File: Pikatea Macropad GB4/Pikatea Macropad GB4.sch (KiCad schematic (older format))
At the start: 30 parts, among them J1 AVR-ISP-6, J2 USB_B_Mini, J3 Conn_01x03_Male, J4 Conn_01x03_Male, J5 Conn_01x03_Male, J6 Conn_01x06_Male, J7 Conn_01x03_Male, SW1 SW_DPST, SW2 Rotary_Encoder_Switch, U1 ATMEGA32U4-EP, X1 16MHz

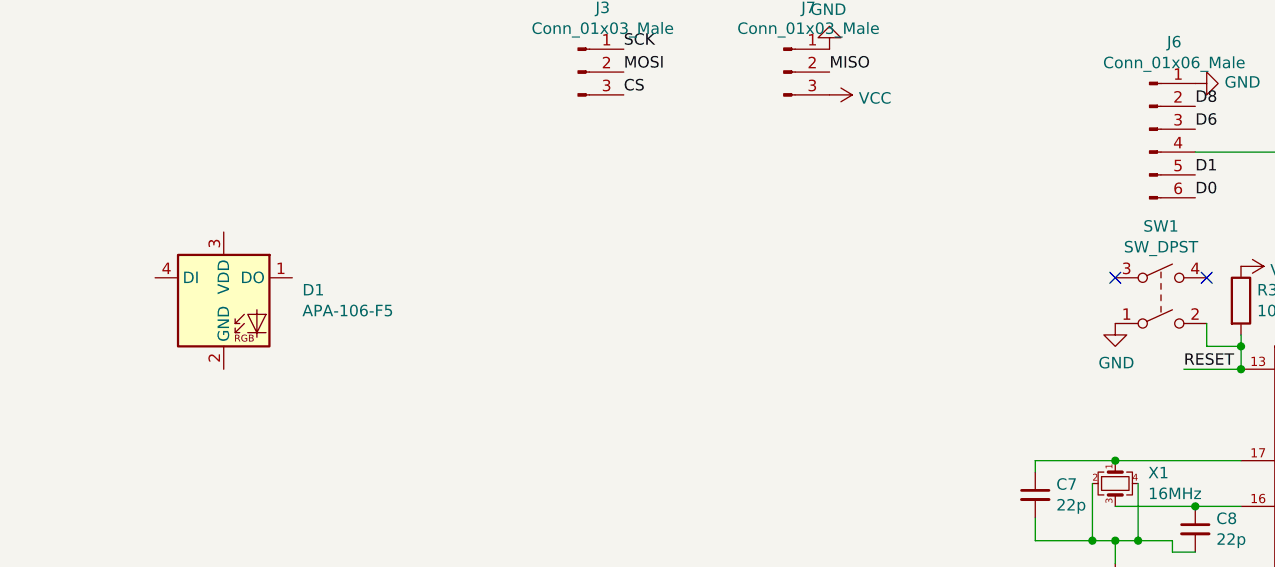
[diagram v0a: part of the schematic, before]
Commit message: update GB4
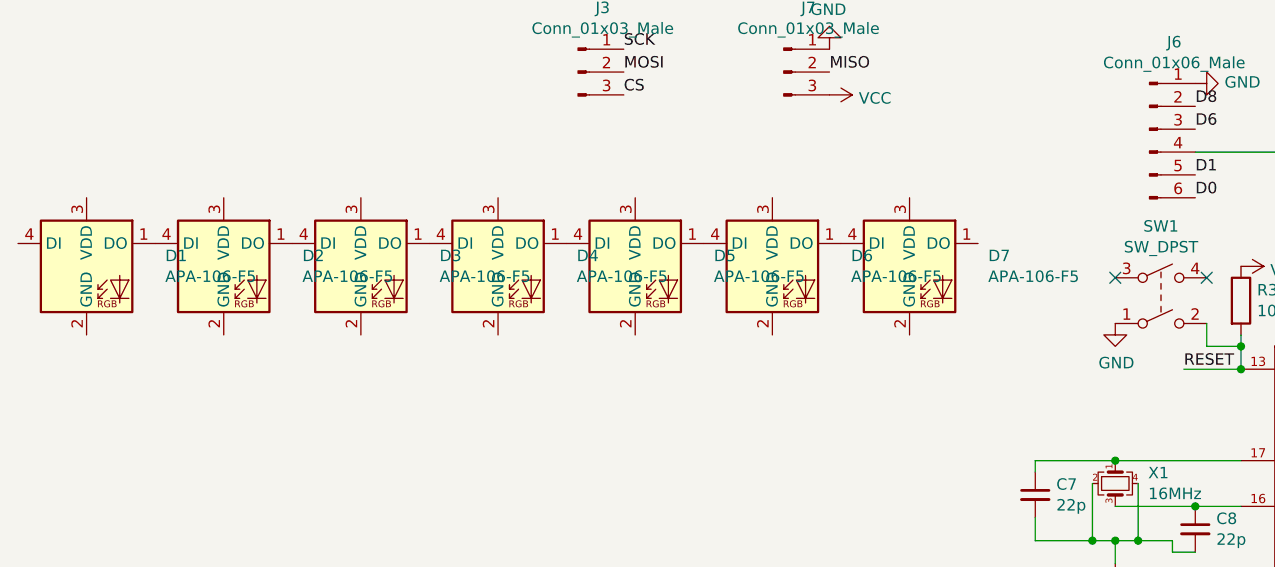
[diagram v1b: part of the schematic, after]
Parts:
- added D2, D3, D4, D5, D6, D7: APA-106-F5, Pikatea:TONYU-DY-S352818-RGBC, symbol LED:APA-106-F5
- D1: footprint LED_THT:LED_D5.0mm-4_RGB -> Pikatea:TONYU-DY-S352818-RGBC
- MX1, MX2, MX3, MX4, MX5: footprint MX_Only:MXOnly-1U -> MX_Only:MXOnly-1U-NoLED
- U1: footprint Package_QFP:LQFP-44_10x10mm_P0.8mm -> Package_DFN_QFN:QFN-44-1EP_7x7mm_P0.5mm_EP5.15x5.15mm_ThermalVias
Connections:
- net at D1.1 (DO): now also D2.4 (DI)
- new net: D2.1 (DO), D3.4 (DI)
- new net: D3.1 (DO), D4.4 (DI)
- new net: D4.1 (DO), D5.4 (DI)
- new net: D5.1 (DO), D6.4 (DI)
- new net: D6.1 (DO), D7.4 (DI)
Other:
- moved on the sheet: D1
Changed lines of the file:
@@
 F 0 "U1" H 7075 6581 50  0000 C CNN
 F 1 "ATMEGA32U4-EP" H 7075 6490 50  0000 C CNN
-F 2 "Package_QFP:LQFP-44_10x10mm_P0.8mm" H 7100 4600 50  0001 C CIN
+F 2 "Package_DFN_QFN:QFN-44-1EP_7x7mm_P0.5mm_EP5.15x5.15mm_ThermalVias" H 7100 4600 50  0001 C CIN
 F 3 "" H 8200 5700 50  0001 C CNN
 	1    7100 4600
@@
 F 0 "MX1" H 7382 2074 60  0000 C CNN
 F 1 "MX-LED" H 7382 2000 20  0000 C CNN
-F 2 "MX_Only:MXOnly-1U" H 6675 1825 60  0001 C CNN
+F 2 "MX_Only:MXOnly-1U-NoLED" H 6675 1825 60  0001 C CNN
 F 3 "" H 6675 1825 60  0001 C CNN
 	1    7300 1850
@@
 F 0 "MX2" H 7832 2074 60  0000 C CNN
 F 1 "MX-LED" H 7832 2000 20  0000 C CNN
-F 2 "MX_Only:MXOnly-1U" H 7125 1825 60  0001 C CNN
+F 2 "MX_Only:MXOnly-1U-NoLED" H 7125 1825 60  0001 C CNN
 F 3 "" H 7125 1825 60  0001 C CNN
 	1    7750 1850
@@
 F 0 "MX3" H 8282 2074 60  0000 C CNN
 F 1 "MX-LED" H 8282 2000 20  0000 C CNN
-F 2 "MX_Only:MXOnly-1U" H 7575 1825 60  0001 C CNN
+F 2 "MX_Only:MXOnly-1U-NoLED" H 7575 1825 60  0001 C CNN
 F 3 "" H 7575 1825 60  0001 C CNN
 	1    8200 1850
@@
 F 0 "MX4" H 8732 2074 60  0000 C CNN
 F 1 "MX-LED" H 8732 2000 20  0000 C CNN
-F 2 "MX_Only:MXOnly-1U" H 8025 1825 60  0001 C CNN
+F 2 "MX_Only:MXOnly-1U-NoLED" H 8025 1825 60  0001 C CNN
 F 3 "" H 8025 1825 60  0001 C CNN
 	1    8650 1850
@@
 F 0 "MX5" H 9182 2074 60  0000 C CNN
 F 1 "MX-LED" H 9182 2000 20  0000 C CNN
-F 2 "MX_Only:MXOnly-1U" H 8475 1825 60  0001 C CNN
+F 2 "MX_Only:MXOnly-1U-NoLED" H 8475 1825 60  0001 C CNN
 F 3 "" H 8475 1825 60  0001 C CNN
 	1    9100 1850
@@
 L LED:APA-106-F5 D1
 U 1 1 61FC7D80
-P 1500 2750
-F 0 "D1" H 1844 2796 50  0000 L CNN
-F 1 "APA-106-F5" H 1844 2705 50  0000 L CNN
-F 2 "LED_THT:LED_D5.0mm-4_RGB" H 1550 2450 50  0001 L TNN
-F 3 "https://cdn.sparkfun.com/datasheets/Components/LED/COM-12877.pdf" H 1600 2375 50  0001 L TNN
-	1    1500 2750
-	1    0    0    -1
-$EndComp
+P 900 2600
+F 0 "D1" H 1244 2646 50  0000 L CNN
+F 1 "APA-106-F5" H 1244 2555 50  0000 L CNN
+F 2 "Pikatea:TONYU-DY-S352818-RGBC" H 950 2300 50  0001 L TNN
+F 3 "https://cdn.sparkfun.com/datasheets/Components/LED/COM-12877.pdf" H 1000 2225 50  0001 L TNN
+	1    900  2600
+	1    0    0    -1
+$EndComp
+$Comp
+L LED:APA-106-F5 D2
+U 1 1 61FFAAD7
+P 1500 2600
+F 0 "D2" H 1844 2646 50  0000 L CNN
+F 1 "APA-106-F5" H 1844 2555 50  0000 L CNN
+F 2 "Pikatea:TONYU-DY-S352818-RGBC" H 1550 2300 50  0001 L TNN
+F 3 "https://cdn.sparkfun.com/datasheets/Components/LED/COM-12877.pdf" H 1600 2225 50  0001 L TNN
+	1    1500 2600
+	1    0    0    -1
+$EndComp
+$Comp
+L LED:APA-106-F5 D3
+U 1 1 61FFB6F5
+P 2100 2600
+F 0 "D3" H 2444 2646 50  0000 L CNN
+F 1 "APA-106-F5" H 2444 2555 50  0000 L CNN
+F 2 "Pikatea:TONYU-DY-S352818-RGBC" H 2150 2300 50  0001 L TNN
+F 3 "https://cdn.sparkfun.com/datasheets/Components/LED/COM-12877.pdf" H 2200 2225 50  0001 L TNN
+	1    2100 2600
+	1    0    0    -1
+$EndComp
+$Comp
+L LED:APA-106-F5 D4
+U 1 1 61FFBE3A
+P 2700 2600
+F 0 "D4" H 3044 2646 50  0000 L CNN
+F 1 "APA-106-F5" H 3044 2555 50  0000 L CNN
+F 2 "Pikatea:TONYU-DY-S352818-RGBC" H 2750 2300 50  0001 L TNN
+F 3 "https://cdn.sparkfun.com/datasheets/Components/LED/COM-12877.pdf" H 2800 2225 50  0001 L TNN
+	1    2700 2600
+	1    0    0    -1
+$EndComp
+$Comp
+L LED:APA-106-F5 D5
+U 1 1 61FFC4C6
+P 3300 2600
+F 0 "D5" H 3644 2646 50  0000 L CNN
+F 1 "APA-106-F5" H 3644 2555 50  0000 L CNN
+F 2 "Pikatea:TONYU-DY-S352818-RGBC" H 3350 2300 50  0001 L TNN
+F 3 "https://cdn.sparkfun.com/datasheets/Components/LED/COM-12877.pdf" H 3400 2225 50  0001 L TNN
+	1    3300 2600
+	1    0    0    -1
+$EndComp
+$Comp
+L LED:APA-106-F5 D6
+U 1 1 61FFCE25
+P 3900 2600
+F 0 "D6" H 4244 2646 50  0000 L CNN
+F 1 "APA-106-F5" H 4244 2555 50  0000 L CNN
+F 2 "Pikatea:TONYU-DY-S352818-RGBC" H 3950 2300 50  0001 L TNN
+F 3 "https://cdn.sparkfun.com/datasheets/Components/LED/COM-12877.pdf" H 4000 2225 50  0001 L TNN
+	1    3900 2600
+	1    0    0    -1
+$EndComp
+$Comp
+L LED:APA-106-F5 D7
+U 1 1 61FFD683
+P 4500 2600
+F 0 "D7" H 4844 2646 50  0000 L CNN
+F 1 "APA-106-F5" H 4844 2555 50  0000 L CNN
+F 2 "Pikatea:TONYU-DY-S352818-RGBC" H 4550 2300 50  0001 L TNN
+F 3 "https://cdn.sparkfun.com/datasheets/Components/LED/COM-12877.pdf" H 4600 2225 50  0001 L TNN
+	1    4500 2600
+	1    0    0    -1
+$EndComp
